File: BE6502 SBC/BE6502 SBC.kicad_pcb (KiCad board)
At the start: 2 copper layers, 99.1 x 99.1 mm, 45 parts, among them J1 Expansion, J2 RC1_UI_Port, J3 BARREL_JACK, J4 K1-4, M1 Mounting, M2 Mounting, M3 Mounting, M4 Mounting, U1 6502, U2 HM62256BLP-7, U3 28C256, U4 6532, U5 74LS00, U6 LM556, U7 74LS138, U8 74LS138, U9 74LS00, X1 1MHz

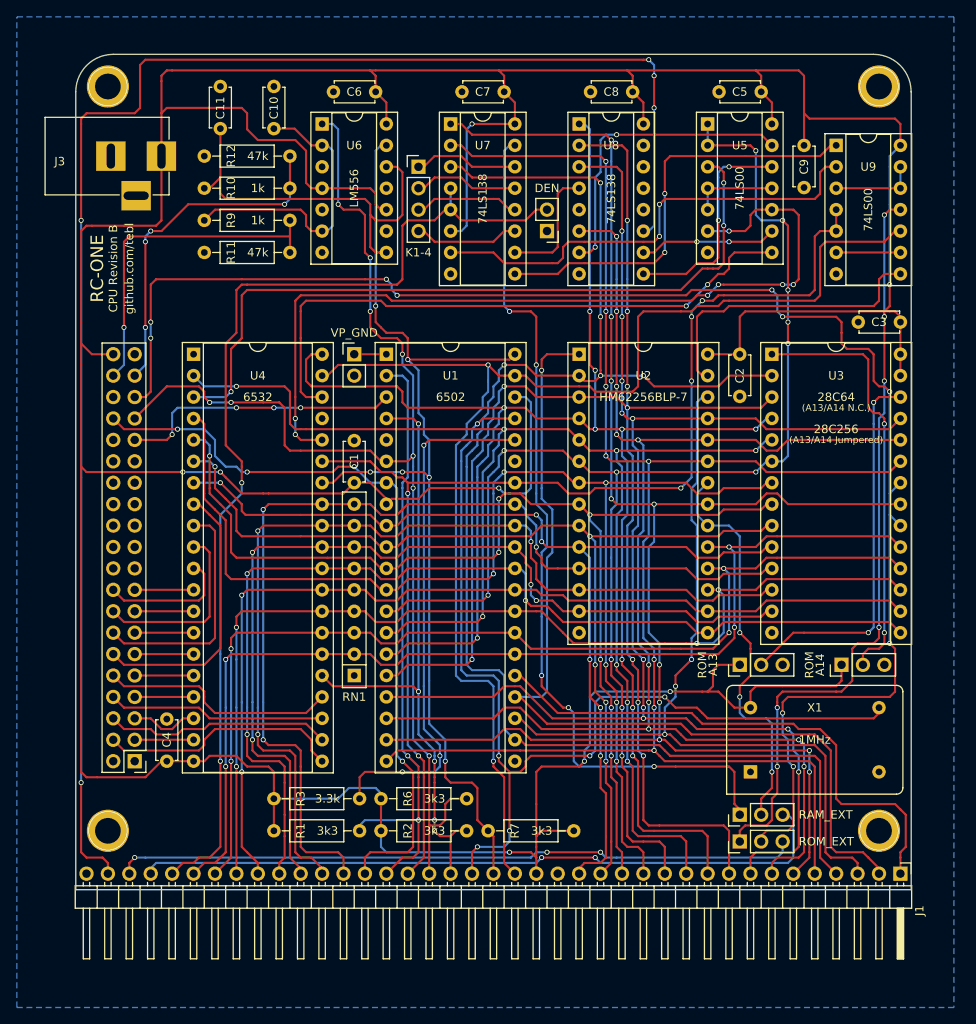
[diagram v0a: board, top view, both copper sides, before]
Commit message: Component placement
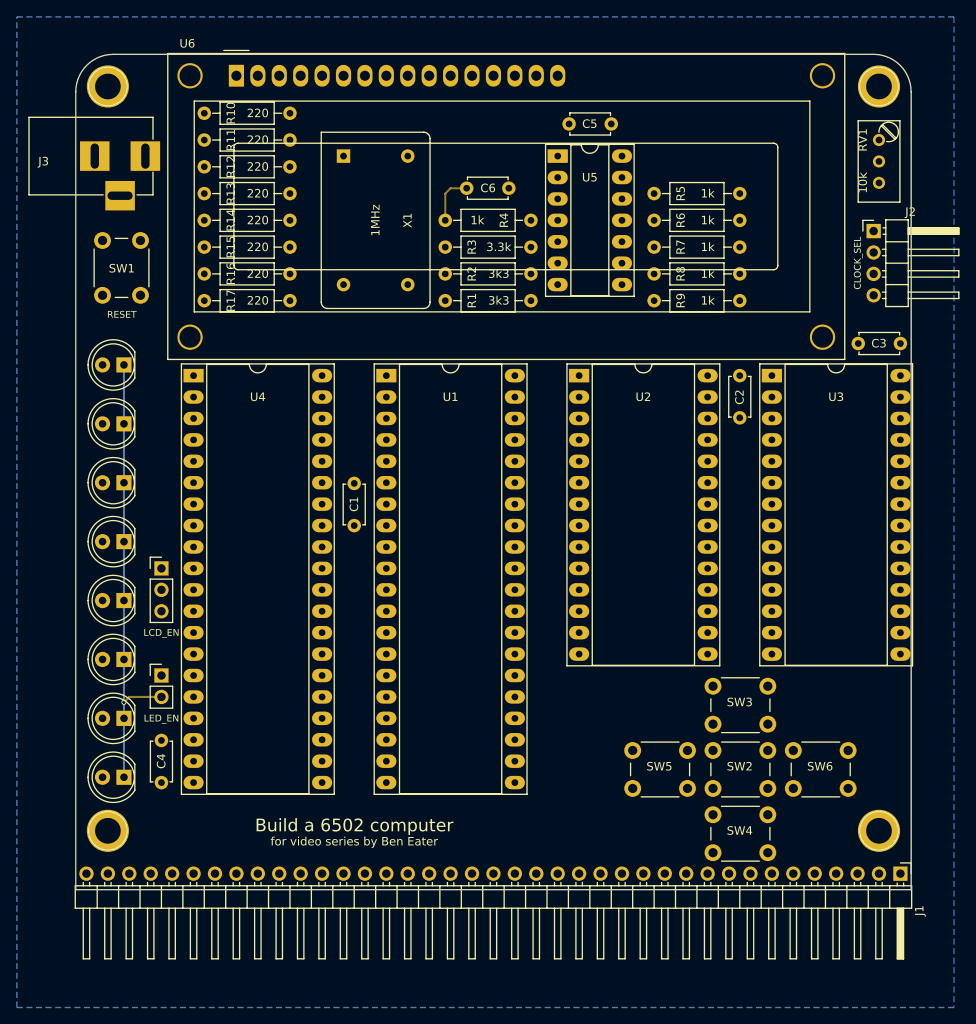
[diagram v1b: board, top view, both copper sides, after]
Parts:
- removed C10, C11: 220nF, Capacitors_THT:C_Disc_D4.7mm_W2.5mm_P5.00mm
- removed C7, C8, C9: 100nF, Capacitors_THT:C_Disc_D4.7mm_W2.5mm_P5.00mm
- removed J4: K1-4, Pin_Headers:Pin_Header_Straight_1x04_Pitch2.54mm
- removed JP3: RAM_CS, Pin_Headers:Pin_Header_Straight_1x03_Pitch2.54mm
- removed JP4: ROM_CS, Pin_Headers:Pin_Header_Straight_1x03_Pitch2.54mm
- removed JP7: A13, Pin_Headers:Pin_Header_Straight_1x03_Pitch2.54mm
- removed JP8: A14, Pin_Headers:Pin_Header_Straight_1x03_Pitch2.54mm
- removed RN1: 4k7x8, Resistors_THT:R_Array_SIP9
- removed U7, U8: 74LS138, Housings_DIP:DIP-16_W7.62mm_Socket
- removed U9: 74LS00, Housings_DIP:DIP-14_W7.62mm_Socket
- added D1: LED, LEDs:LED_D5.0mm, F.Cu at (106.0, 85.1)
- added D2: LED, LEDs:LED_D5.0mm, F.Cu at (106.0, 92.1)
- added D3: LED, LEDs:LED_D5.0mm, F.Cu at (106.0, 99.1)
- added D4: LED, LEDs:LED_D5.0mm, F.Cu at (106.0, 106.0)
- added D5: LED, LEDs:LED_D5.0mm, F.Cu at (106.0, 113.0)
- added D6: LED, LEDs:LED_D5.0mm, F.Cu at (106.0, 120.0)
- added D7: LED, LEDs:LED_D5.0mm, F.Cu at (106.0, 127.0)
- added D8: LED, LEDs:LED_D5.0mm, F.Cu at (106.0, 134.0)
- added R13: 220, Resistors_THT:R_Axial_DIN0207_L6.3mm_D2.5mm_P10.16mm_Horizontal, F.Cu at (115.6, 64.8)
- added R14: 220, Resistors_THT:R_Axial_DIN0207_L6.3mm_D2.5mm_P10.16mm_Horizontal, F.Cu at (115.6, 67.9)
- added R15: 220, Resistors_THT:R_Axial_DIN0207_L6.3mm_D2.5mm_P10.16mm_Horizontal, F.Cu at (115.6, 71.1)
- added R16: 220, Resistors_THT:R_Axial_DIN0207_L6.3mm_D2.5mm_P10.16mm_Horizontal, F.Cu at (115.6, 74.3)
- added R17: 220, Resistors_THT:R_Axial_DIN0207_L6.3mm_D2.5mm_P10.16mm_Horizontal, F.Cu at (115.6, 77.5)
- added R4: 1k, Resistors_THT:R_Axial_DIN0207_L6.3mm_D2.5mm_P10.16mm_Horizontal, F.Cu at (154.3, 67.9)
- added R5: 1k, Resistors_THT:R_Axial_DIN0207_L6.3mm_D2.5mm_P10.16mm_Horizontal, F.Cu at (168.9, 64.8)
- added R8: 1k, Resistors_THT:R_Axial_DIN0207_L6.3mm_D2.5mm_P10.16mm_Horizontal, F.Cu at (168.9, 74.3)
- added RV1: 10k, Potentiometers:Potentiometer_Trimmer_Bourns_3296W, F.Cu at (195.6, 58.4)
- added SW1: RESET, Buttons_Switches_THT:SW_PUSH_6mm, F.Cu at (103.5, 76.8)
- added SW2: MIDDLE, Buttons_Switches_THT:SW_PUSH_6mm, F.Cu at (175.9, 130.8)
- added SW3: UP, Buttons_Switches_THT:SW_PUSH_6mm, F.Cu at (175.9, 123.2)
- added SW4: DOWN, Buttons_Switches_THT:SW_PUSH_6mm, F.Cu at (175.9, 138.4)
- added SW5: LEFT, Buttons_Switches_THT:SW_PUSH_6mm, F.Cu at (166.4, 130.8)
- added SW6: RIGHT, Buttons_Switches_THT:SW_PUSH_6mm, F.Cu at (185.4, 130.8)
- J2: value RC1_UI_Port -> CLOCK_SEL; footprint Pin_Headers:Pin_Header_Straight_2x20_Pitch2.54mm -> Pin_Headers:Pin_Header_Angled_1x04_Pitch2.54mm
- JP1: value VP_GND -> LED_EN
- JP2: value DEN -> LCD_EN; footprint Pin_Headers:Pin_Header_Straight_1x02_Pitch2.54mm -> Pin_Headers:Pin_Header_Straight_1x03_Pitch2.54mm
- R10: value 1k -> 220
- R11, R12: value 47k -> 220
- R6, R7: value 3k3 -> 1k
- U1: value 6502 -> W65C02; footprint Housings_DIP:DIP-40_W15.24mm_Socket -> Housings_DIP:DIP-40_W15.24mm_Socket_LongPads
- U2, U3: footprint Housings_DIP:DIP-28_W15.24mm_Socket -> Housings_DIP:DIP-28_W15.24mm_Socket_LongPads
- U4: value 6532 -> WD65C22; footprint Housings_DIP:DIP-40_W15.24mm_Socket -> Housings_DIP:DIP-40_W15.24mm_Socket_LongPads
- U5: value 74LS00 -> 74HC00; footprint Housings_DIP:DIP-14_W7.62mm_Socket -> Housings_DIP:DIP-14_W7.62mm_Socket_LongPads
- U6: value LM556 -> RC1602A; footprint Housings_DIP:DIP-14_W7.62mm_Socket -> Displays:WC1602A
- moved J2 107.8 mm to (194.9, 69.2), turned to 0 degrees
- moved X1 87.5 mm to (132.1, 60.3), turned to 270 degrees
- moved R6 72.1 mm to (168.9, 67.9), turned to 0 degrees
- moved R7 72.0 mm to (168.9, 71.1)
- moved R3 68.5 mm to (154.3, 71.1)
- moved R2 66.5 mm to (154.3, 74.3)
- moved R1 66.1 mm to (154.3, 77.5)
- moved JP2 60.8 mm to (110.5, 109.2), turned to 0 degrees
- moved R9 54.2 mm to (168.9, 77.5)
- moved JP1 44.4 mm to (110.5, 121.9)
- moved C5 18.2 mm to (163.8, 56.5)
- moved U5 18.2 mm to (157.5, 60.3)
- moved C6 15.7 mm to (146.7, 64.1), turned to 0 degrees
- moved R11 13.3 mm to (115.6, 58.4)
- moved U6 11.7 mm to (119.4, 50.8)
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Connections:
- C6 pad 1: VCC -> ~RESET
- J1 pad 19: /PHI2 -> CLOCK
- J1 pad 20: /~RESET -> ~RESET
- J1 pad 21: /PHI0 -> (no net)
- J1 pad 35: /DEN -> (no net)
- J1 pad 36: K0_EXT -> (no net)
- J1 pad 37: K7_EXT -> (no net)
- J1 pad 38: ~IO3 -> (no net)
- J2 pad 1: GND -> VCC
- J2 pad 2: GND -> Net-(J2-Pad2)
- J2 pad 3: /PB4 -> CLOCK
- J2 pad 4: /PB3 -> GND
- JP1 pad 1: Net-(JP1-Pad1) -> GND
- JP1 pad 2: GND -> Net-(D1-Pad1)
- JP2 pad 1: GND -> /PA7
- JP2 pad 2: /DEN -> Net-(JP2-Pad2)
- R10 pad 1: Net-(C11-Pad2) -> Net-(D1-Pad2)
- R10 pad 2: RS -> /PB0
- R11 pad 1: GND -> Net-(D2-Pad2)
- R11 pad 2: ST -> /PB1
- R12 pad 1: GND -> Net-(D3-Pad2)
- R12 pad 2: RS -> /PB2
- R3 pad 1: /BE -> /~NMI
- R6 pad 1: /~NMI -> VCC
- R6 pad 2: VCC -> /PA1
- R7 pad 1: /~RESET -> VCC
- R7 pad 2: VCC -> /PA2
- R9 pad 1: Net-(C10-Pad2) -> VCC
- R9 pad 2: ST -> /PA4
- U1 pad 1: Net-(JP1-Pad1) -> (no net)
- U1 pad 3: /PHI1 -> (no net)
- U1 pad 36: /BE -> (no net)
- U1 pad 37: /PHI0 -> CLOCK
- U1 pad 38: VCC -> (no net)
- U1 pad 39: /PHI2 -> (no net)
- U1 pad 40: /~RESET -> ~RESET
- U2 pad 20: K0 -> ~RAM
- U2 pad 22: K0 -> /A14
- U2 pad 27: RAM_R/~W -> /R/~W
- U3 pad 1: Net-(JP8-Pad2) -> /A14
- U3 pad 20: K7 -> ~ROM
- U3 pad 22: K7 -> GND
- U3 pad 26: Net-(JP7-Pad2) -> /A13
- U4 pad 10: /PA2 -> /PB0
- U4 pad 11: /PA3 -> /PB1
- U4 pad 12: /PA4 -> /PB2
- U4 pad 13: /PA5 -> /PB3
- U4 pad 14: /PA6 -> /PB4
- U4 pad 15: /PA7 -> /PB5
- U4 pad 16: /PB7 -> /PB6
- U4 pad 17: /PB6 -> /PB7
- U4 pad 18: /PB5 -> (no net)
- U4 pad 19: /PB4 -> (no net)
- U4 pad 2: /A5 -> /PA0
- U4 pad 21: /PB3 -> /~IRQ
- U4 pad 22: /PB2 -> /R/~W
- U4 pad 23: /PB1 -> ~VIA
- U4 pad 24: /PB0 -> /A13
- U4 pad 25: /~IRQ -> CLOCK
- U4 pad 3: /~A4 -> /PA1
- U4 pad 34: /~RESET -> ~RESET
- U4 pad 35: /R/~W -> /A3
- U4 pad 36: ~RAM_SEL -> /A2
- U4 pad 37: GND -> /A1
- U4 pad 38: IO2 -> /A0
- U4 pad 39: /PHI2 -> (no net)
- U4 pad 4: /A3 -> /PA2
- U4 pad 40: /A6 -> (no net)
- U4 pad 5: /A2 -> /PA3
- U4 pad 6: /A1 -> /PA4
- U4 pad 7: /A0 -> /PA5
- U4 pad 8: /PA0 -> /PA6
- U4 pad 9: /PA1 -> /PA7
- U5 pad 1: /A4 -> GND
- U5 pad 10: ~RAM_SEL -> ~ROM
- U5 pad 11: Net-(U5-Pad11) -> ~ROM
- U5 pad 12: Net-(U5-Pad12) -> /A15
- U5 pad 13: Net-(U5-Pad13) -> /A15
- U5 pad 2: /A4 -> GND
- U5 pad 3: /~A4 -> (no net)
- U5 pad 4: Net-(U5-Pad11) -> ~ROM
- U5 pad 5: Net-(U5-Pad11) -> /A14
- U5 pad 6: ~RAM_SEL -> ~VIA
- U5 pad 8: IO2 -> ~RAM
- U5 pad 9: Net-(U5-Pad9) -> CLOCK
- U6 pad 1: /~NMI -> GND
- U6 pad 10: VCC -> /PB3
- U6 pad 11: (no net) -> /PB4
- U6 pad 12: Net-(C11-Pad2) -> /PB5
- U6 pad 13: /~RESET -> /PB6
- U6 pad 14: VCC -> /PB7
- U6 pad 2: Net-(C10-Pad2) -> VCC
- U6 pad 3: (no net) -> Net-(RV1-Pad2)
- U6 pad 4: VCC -> /PA5
- U6 pad 5: (no net) -> /PA6
- U6 pad 6: Net-(C10-Pad2) -> Net-(JP2-Pad2)
- U6 pad 7: GND -> /PB0
- U6 pad 8: Net-(C11-Pad2) -> /PB1
- U6 pad 9: (no net) -> /PB2
- X1 pad 8: /PHI0 -> Net-(J2-Pad2)
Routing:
- net VCC: track 548.6 -> 0.00 mm, vias 8 -> 0
- net /A6: track 202.7 -> 0.00 mm, vias 10 -> 0
- net /A10: track 195.1 -> 0.00 mm, vias 10 -> 0
- net /A11: track 190.3 -> 0.00 mm, vias 8 -> 0
- net K7: track 187.7 -> 0.00 mm, vias 10 -> 0
- net ~IO3: track 187.3 -> 0.00 mm, vias 5 -> 0
- net /A7: track 180.7 -> 0.00 mm, vias 9 -> 0
- net /A12: track 177.8 -> 0.00 mm, vias 5 -> 0
- net /A8: track 177.8 -> 0.00 mm, vias 10 -> 0
- net /A9: track 168.7 -> 0.00 mm, vias 10 -> 0
- net /A5: track 168.2 -> 0.00 mm, vias 8 -> 0
- net /A4: track 167.1 -> 0.00 mm, vias 12 -> 0
- net /PHI2: track 153.2 -> 0.00 mm, vias 2 -> 0
- net /A3: track 148.6 -> 0.00 mm, vias 6 -> 0
- net /~NMI: track 145.5 -> 0.00 mm, vias 9 -> 0
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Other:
- board text added: "6522 VIA"
- board text added: "BE6502"
- board text added: "Build a 6502 computer"
- board text added: "SBC Revision A"
- board text added: "for video series by Ben Eater"
- board text removed: "$0000 - $03FF"
- board text removed: "$0000 - $1FFF OPTIONAL $2000 - $3FFF $4000 - $5FFF $6000 - $7FFF"
- board text removed: "$1740 $1741 $1742 $1743"
- board text removed: "$1740 - $17FF"
- board text removed: "$1744 $1745 $1746 $1747"
- board text removed: "$174C $174D $174E $174F"
- board text removed: "$1780 - $17FF"
- board text removed: "$1800 - $FFFF"
- board text removed: "$E000 - $FFFF"
- board text removed: "$FFFA $17FA $FFFC $FFFE $17FE"
- board text removed: "$FFFB $17FB $FFFD $FFFF $17FF"
- board text removed: "(A13/A14 Jumpered)"
- board text removed: "(A13/A14 N.C.)"
- board text removed: "/1 /8 /64 /1024"
- board text removed: "/1 int. /8 int. /64 int. /1024 int."
- board text removed: "1-2 Standalone 2-3 65K Expansion"
- board text removed: "28C64"
- board text removed: "6532 RIOT"
- board text removed: "65K EXPANSION"
- board text removed: "8K0"
- board text removed: "A13"
- board text removed: "A14"
- board text removed: "ADDRESS DECODER"
- board text removed: "CPU Revision B"
- board text removed: "INTERRUPT"
- board text removed: "K5"
- board text removed: "MEMORY DECODING"
- board text removed: "NMI RST IRQ"
- board text removed: "Port A Port A DDR Port B Port B DDR"
- board text removed: "RAM_EXT"
- board text removed: "RC-ONE"
- board text removed: "REGISTERS"
- board text removed: "ROM"
- board text removed: "ROM_EXT"
- board text removed: "SWITCH DEBOUNCE"
- board text removed: "TIMER"
- board text removed: "VECTORS"
